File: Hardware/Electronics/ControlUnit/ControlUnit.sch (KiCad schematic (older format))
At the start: 78 parts, among them J1 Screw_Terminal_01x02, Batt 9V, J10 S3, J11 MPU-6050/MPU-9250, J12 S4, J13 Conn_01x02, J2 USB_B_Mini, J3 Conn_01x05, J4 Conn_Coaxial, J5 Conn_Coaxial, J6 Micro_SD_Card, J7 S1, J8 BME280, J9 S2, Q1 , Q2 , SW1 SW_DPDT_x2, SW2 SW_Push, U1 ATSAMD21G18A-AFT, U2 LM340_SOT223/LM7805_5V, U3 MCP1826S_3.3V, U4 RFM69W, U5 MAX-8Q, U6 W25Q32JVSS, Y1 32.768kHz

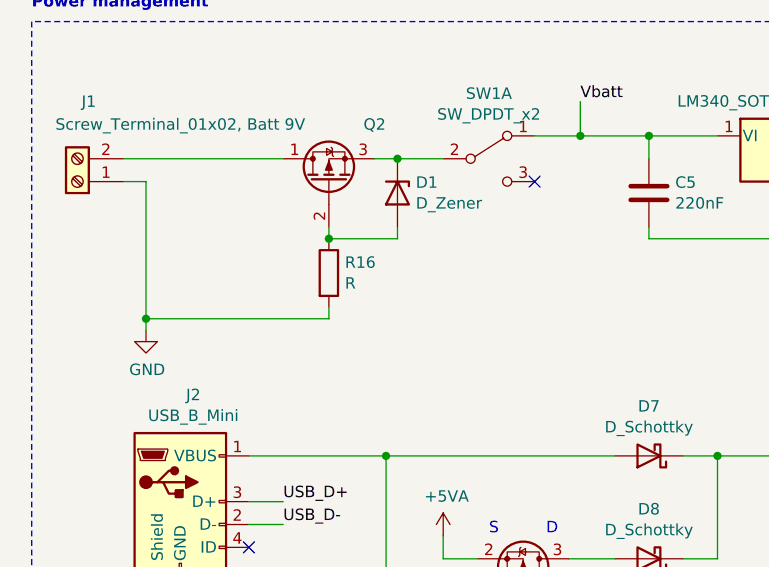
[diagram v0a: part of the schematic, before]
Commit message: Encore
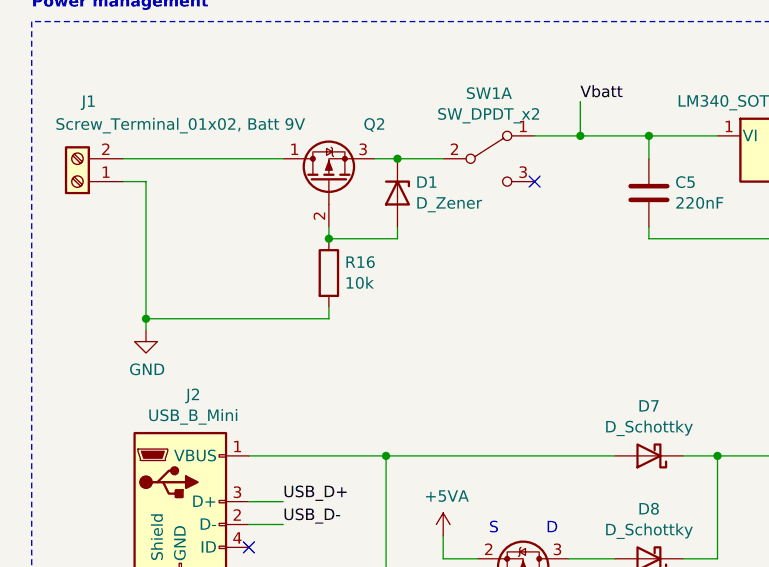
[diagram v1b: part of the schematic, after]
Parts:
- R16: value R -> 10k
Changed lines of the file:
@@
 P 2250 8500
 F 0 "R16" H 2320 8546 50  0000 L CNN
-F 1 "R" H 2320 8455 50  0000 L CNN
+F 1 "10k" H 2320 8455 50  0000 L CNN
 F 2 "" V 2180 8500 50  0001 C CNN
 F 3 "~" H 2250 8500 50  0001 C CNN
